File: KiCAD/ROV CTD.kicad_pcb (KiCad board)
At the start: 2 copper layers, 73.7 x 23.4 mm, 36 parts, among them J10 1Wire1, J11 1Wire2, J12 1Wire3, J4 Bottom - Middle, J6 Main In, J7 Bottom - Middle, J8 Middle - Top, J9 Middle - Top, U1 EZO-EC, U2 ATtiny1614-Arduino, U3 AP63205WU, U6 MAX3072E

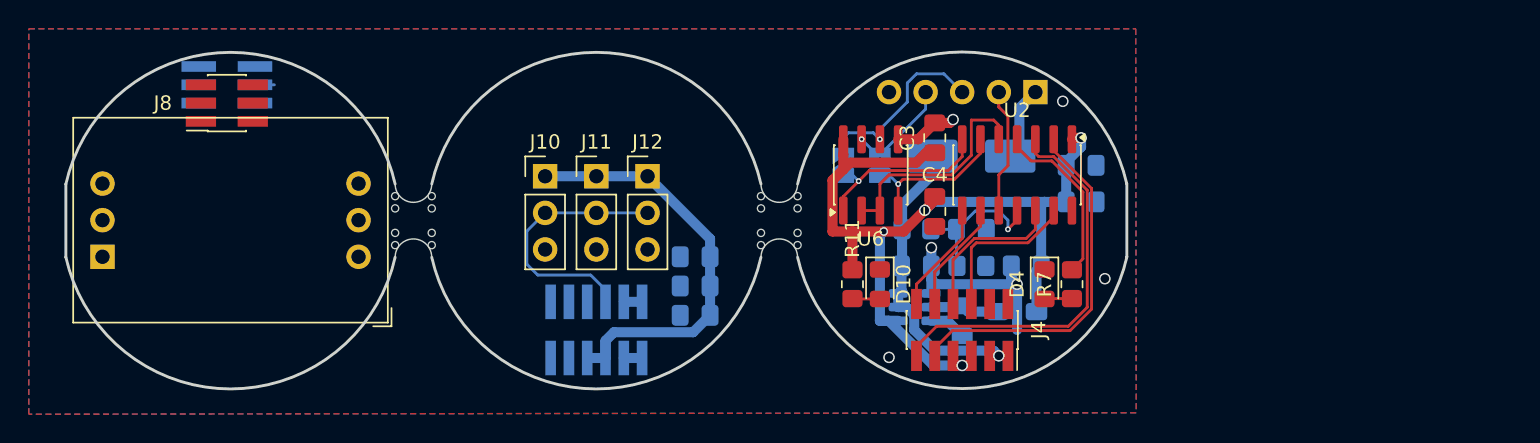
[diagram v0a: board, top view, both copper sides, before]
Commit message: .
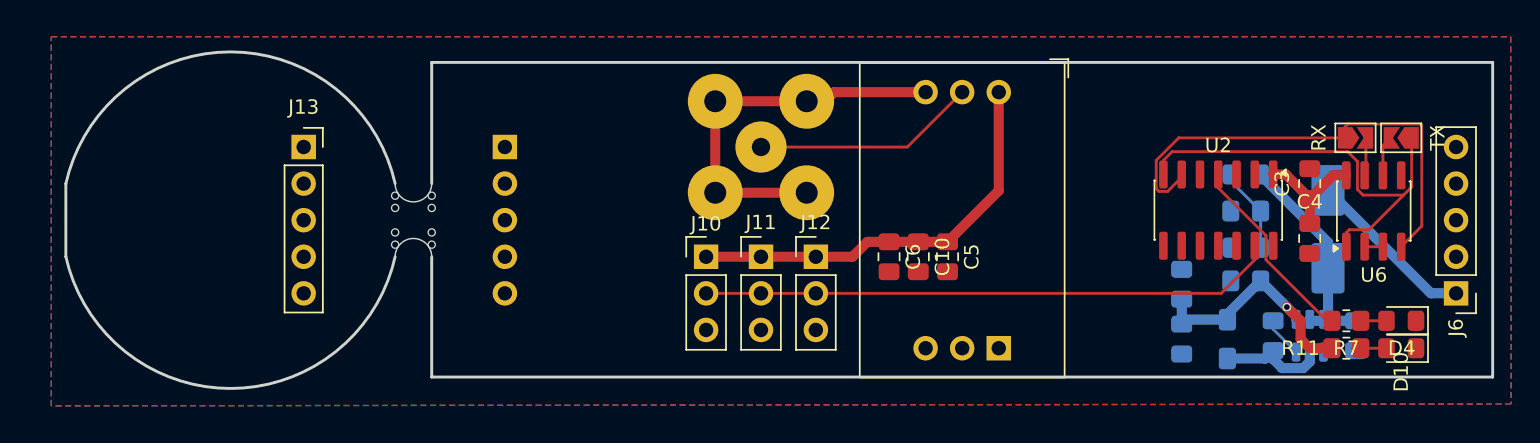
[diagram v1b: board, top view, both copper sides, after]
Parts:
- removed J4: Bottom - Middle, Connector_PinSocket_1.27mm:PinSocket_2x06_P1.27mm_Vertical_SMD
- removed J7: Bottom - Middle, Connector_PinHeader_1.27mm:PinHeader_2x06_P1.27mm_Vertical_SMD
- removed J8: Middle - Top, Connector_PinSocket_1.27mm:PinSocket_2x03_P1.27mm_Vertical_SMD
- removed J9: Middle - Top, Connector_PinHeader_1.27mm:PinHeader_2x03_P1.27mm_Vertical_SMD
- removed the REF** at (179.1, 76.2)
- removed the REF** at (165.1, 71.1)
- removed U1: EZO-EC, KiCad Footprints:EZO_Conductivity_Module
- added J1: Conn_Coaxial, Connector_Coaxial:BNC_TEConnectivity_1478204_Vertical, B.Cu at (176.5, 71.1)
- added J13: Interface, Connector_PinSocket_2.54mm:PinSocket_1x05_P2.54mm_Vertical, F.Cu at (144.8, 71.1)
- added J14: Interface, Connector_PinHeader_2.54mm:PinHeader_1x05_P2.54mm_Horizontal, B.Cu at (158.8, 71.1)
- added M1: EZO-EC, KiCad Footprints:EZO_Conductivity_Module, F.Cu at (190.5, 76.2)
- C10, C5, C6, J6, JP1, JP2: moved to F.Cu
- moved JP1 38.8 mm to (221.0, 70.5), turned to 180 degrees
- moved D10 36.5 mm to (221.0, 85.1), turned to 180 degrees
- moved U6 35.0 mm to (219.1, 75.6)
- moved R11 34.6 mm to (217.2, 85.1), turned to 0 degrees
- moved JP2 33.1 mm to (217.8, 70.5), turned to 0 degrees
- moved J6 32.4 mm to (224.8, 81.3), turned to 180 degrees
- moved C14 30.9 mm to (217.8, 84.2), turned to 90 degrees
- moved U3 27.5 mm to (214.6, 84.2), turned to -90 degrees
- moved C3 26.2 mm to (214.6, 73.7)
- moved C4 26.1 mm to (214.6, 77.5)
- moved D5 25.3 mm to (215.9, 76.8), turned to 90 degrees
- moved D4 24.9 mm to (221.0, 83.2), turned to 180 degrees
- moved R9 23.2 mm to (210.2, 73.0), turned to 180 degrees
- moved C15 21.6 mm to (212.1, 84.2), turned to 90 degrees
- moved R7 19.2 mm to (217.2, 83.2), turned to 0 degrees
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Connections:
- C10 pad 1: +5V_Mid -> +5V
- C5 pad 1: +5V_Mid -> +5V
- C6 pad 1: +5V_Mid -> +5V
- J10 pad 1: +5V_Mid -> +5V
- J11 pad 1: +5V_Mid -> +5V
- J12 pad 1: +5V_Mid -> +5V
- U2 pad 13: /NeoPixle -> /1Wire
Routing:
- net +5V_Mid: track 29.0 -> 0.00 mm
- net Net-(J1-Ext): track 0.00 -> 27.6 mm
- net /STATUS_LED: track 26.8 -> 0.00 mm
- net /LED_PWM: track 24.1 -> 0.00 mm
- net /SERIAL_RX: track 10.9 -> 33.4 mm, vias 1 -> 0
- net /1Wire: track 18.2 -> 40.0 mm
- net GND: track 19.5 -> 0.00 mm, vias 6 -> 0
- net /SERIAL_TX: track 12.8 -> 30.5 mm, vias 1 -> 0
- net /SERIAL_DIR: track 15.8 -> 1.27 mm
- net Net-(J1-In): track 0.00 -> 14.3 mm
- net /NeoPixle: track 12.3 -> 0.00 mm
- net /A9/D9: track 11.0 -> 0.00 mm
- net /Data_A: track 13.3 -> 2.83 mm, vias 1 -> 0
- net +5V: track 63.5 -> 54.4 mm, vias 4 -> 1
- net /UPDI: track 8.75 -> 0.00 mm
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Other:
- board size 73.7 x 23.4 mm -> 99.1 x 23.4 mm
